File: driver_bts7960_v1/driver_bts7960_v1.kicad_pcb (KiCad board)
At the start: 2 copper layers, 56.5 x 43.7 mm, 31 parts, among them J1 Motor_1, J2 Alimentacion, J6 Motor_2, J7 Conn_02x04_Odd_Even, U1 BTS7960B, U2 BTS7960B, U3 BTS7960B, U4 BTS7960B

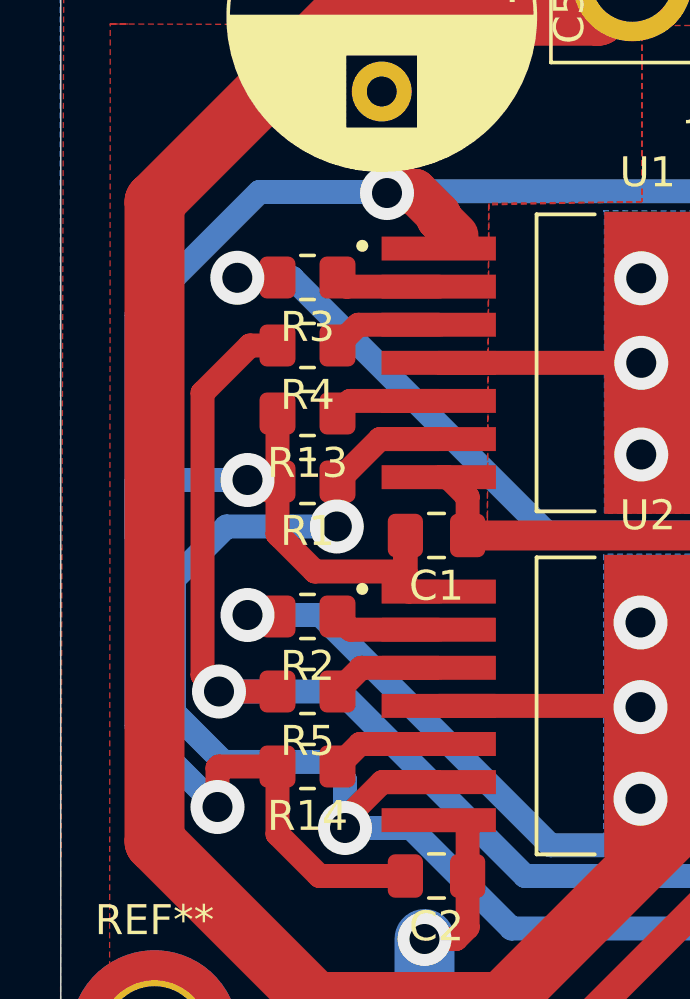
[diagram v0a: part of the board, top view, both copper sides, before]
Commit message: .
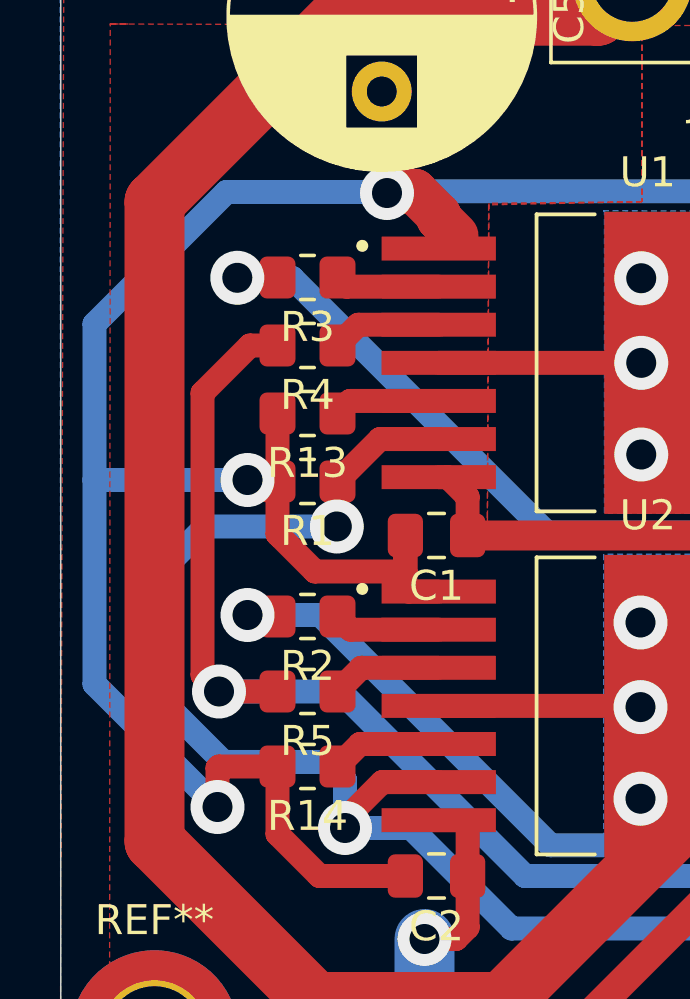
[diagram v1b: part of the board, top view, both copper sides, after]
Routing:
- net GND: track 171.3 -> 172.7 mm
- net IS_1: track 43.7 -> 44.7 mm
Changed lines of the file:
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@@
-	)
-	(segment
-		(start 127.951 69.496115)
-		(end 127.951 76.9)
-		(width 0.8)
-		(layer "B.Cu")
-		(net 1)
 	)
 	(segment
@@
 	)
 	(segment
+		(start 126.55 69.8)
+		(end 126.55 81.8)
+		(width 0.8)
+		(layer "B.Cu")
+		(net 1)
+	)
+	(segment
 		(start 173.75 76.85)
 		(end 172.35 76.85)
@@
 	)
 	(segment
+		(start 136.3 65.434246)
+		(end 136.265754 65.4)
+		(width 0.8)
+		(layer "B.Cu")
+		(net 1)
+	)
+	(segment
+		(start 136.265754 65.4)
+		(end 130.95 65.4)
+		(width 0.8)
+		(layer "B.Cu")
+		(net 1)
+	)
+	(segment
 		(start 171.8 76.3)
 		(end 171.8 71.55)
@@
 	)
 	(segment
-		(start 132.047115 65.4)
-		(end 127.951 69.496115)
-		(width 0.8)
-		(layer "B.Cu")
-		(net 1)
-	)
-	(segment
 		(start 171.8 71.55)
 		(end 172.95 70.4)
@@
 	)
 	(segment
-		(start 130.65 85.9)
-		(end 127.951 83.201)
-		(width 0.8)
-		(layer "B.Cu")
-		(net 1)
-	)
-	(segment
-		(start 136.3 65.434246)
-		(end 136.265754 65.4)
+		(start 130.95 65.4)
+		(end 126.55 69.8)
 		(width 0.8)
 		(layer "B.Cu")
@@
 	)
 	(segment
-		(start 136.265754 65.4)
-		(end 132.047115 65.4)
-		(width 0.8)
-		(layer "B.Cu")
-		(net 1)
-	)
-	(segment
-		(start 127.951 83.201)
-		(end 127.951 76.9)
+		(start 126.55 81.8)
+		(end 130.65 85.9)
 		(width 0.8)
 		(layer "B.Cu")
@@
 	(segment
 		(start 131.651 75)
-		(end 128.001 75)
-		(width 0.8)
-		(layer "B.Cu")
-		(net 1)
-	)
-	(segment
-		(start 127.951 75.05)
-		(end 127.951 76.9)
+		(end 126.55 75)
 		(width 0.8)
 		(layer "B.Cu")
@@
 		(start 172.35 76.85)
 		(end 171.8 76.3)
-		(width 0.8)
-		(layer "B.Cu")
-		(net 1)
-	)
-	(segment
-		(start 128.001 75)
-		(end 127.951 75.05)
 		(width 0.8)
 		(layer "B.Cu")
@@
 	)
 	(segment
-		(start 130.95 76.55)
-		(end 129.199 78.301)
+		(start 134.299 84.399)
+		(end 134.9 85)
+		(width 0.8)
+		(layer "B.Cu")
+		(net 7)
+	)
+	(segment
+		(start 134.627187 76.55)
+		(end 130.25 76.55)
+		(width 0.8)
+		(layer "B.Cu")
+		(net 7)
+	)
+	(segment
+		(start 148.97 89.95)
+		(end 140.45 89.95)
+		(width 0.8)
+		(layer "B.Cu")
+		(net 7)
+	)
+	(segment
+		(start 137.1 86.6)
+		(end 134.9 86.6)
+		(width 0.8)
+		(layer "B.Cu")
+		(net 7)
+	)
+	(segment
+		(start 128.475 78.325)
+		(end 128.475 82.024)
 		(width 0.8)
 		(layer "B.Cu")
@@
 	)
 	(segment
-		(start 134.627187 76.55)
-		(end 130.95 76.55)
-		(width 0.8)
-		(layer "B.Cu")
-		(net 7)
-	)
-	(segment
-		(start 134.299 84.399)
-		(end 134.9 85)
-		(width 0.8)
-		(layer "B.Cu")
-		(net 7)
-	)
-	(segment
-		(start 148.97 89.95)
-		(end 140.45 89.95)
-		(width 0.8)
-		(layer "B.Cu")
-		(net 7)
-	)
-	(segment
-		(start 129.199 78.301)
-		(end 129.199 82.748)
-		(width 0.8)
-		(layer "B.Cu")
-		(net 7)
-	)
-	(segment
-		(start 137.1 86.6)
-		(end 134.9 86.6)
-		(width 0.8)
-		(layer "B.Cu")
-		(net 7)
-	)
-	(segment
-		(start 129.199 82.748)
+		(start 140.45 89.95)
+		(end 137.1 86.6)
+		(width 0.8)
+		(layer "B.Cu")
+		(net 7)
+	)
+	(segment
+		(start 128.475 82.024)
 		(end 130.85 84.399)
+		(width 0.8)
+		(layer "B.Cu")
+		(net 7)
+	)
+	(segment
+		(start 130.25 76.55)
+		(end 128.475 78.325)
 		(width 0.8)
 		(layer "B.Cu")
@@
 		(width 0.8)
 		(layer "B.Cu")
-		(net 7)
-	)
-	(segment
-		(start 140.45 89.95)
-		(end 137.1 86.6)
-		(width 0.8)
-		(layer "B.Cu")
